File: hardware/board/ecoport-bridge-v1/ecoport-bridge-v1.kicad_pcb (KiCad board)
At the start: 2 copper layers, 51.5 x 92 mm, 68 parts, among them J1 420B2V12FL0, J2 Conn_01x02, J3 SM04B-SRSS-TB, J4 USB4085-GF-A, J5 Conn_01x02, J6 Connector Wire, J7 B3B-PH-K-S, SW1 RESET, SW2 BOOT, U1 IRM-05-5, U2 TLV75733PDBVR, U3 SP3485EET, U4 USBLC6-2SC6, U5 SN74LV1T34DCKR, U6 ESP32-C6-WROOM-1-N8, U7 USBLC6-2SC6

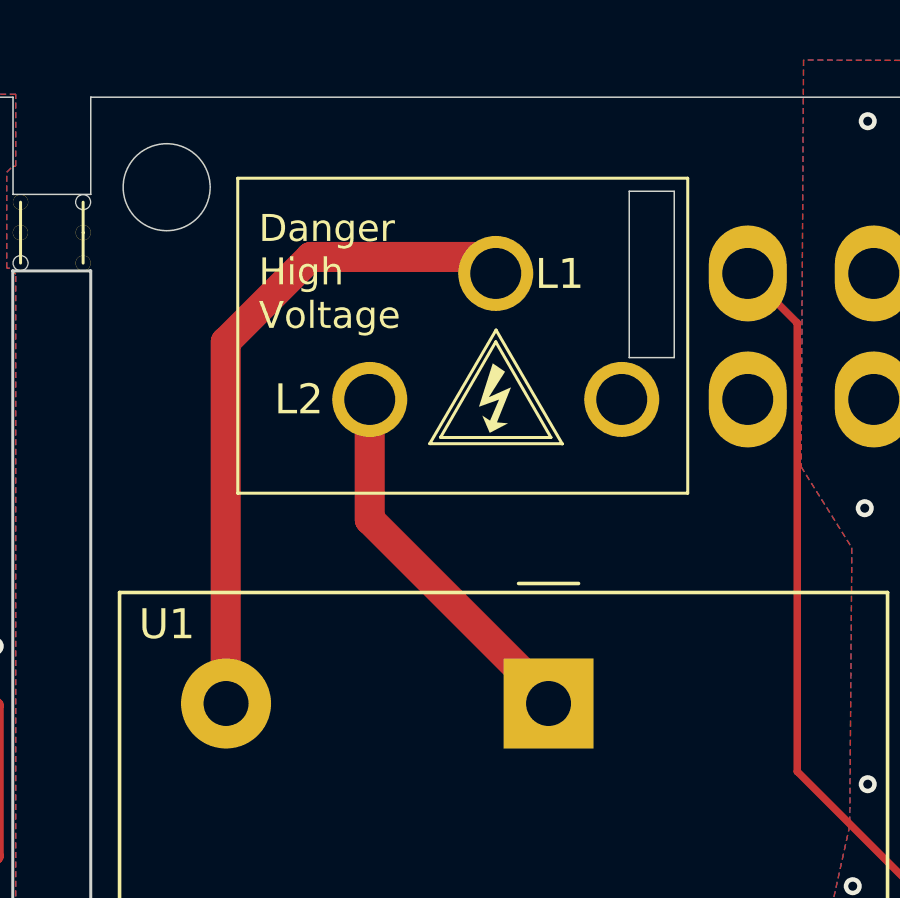
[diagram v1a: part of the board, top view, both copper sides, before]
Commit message: Added fuse
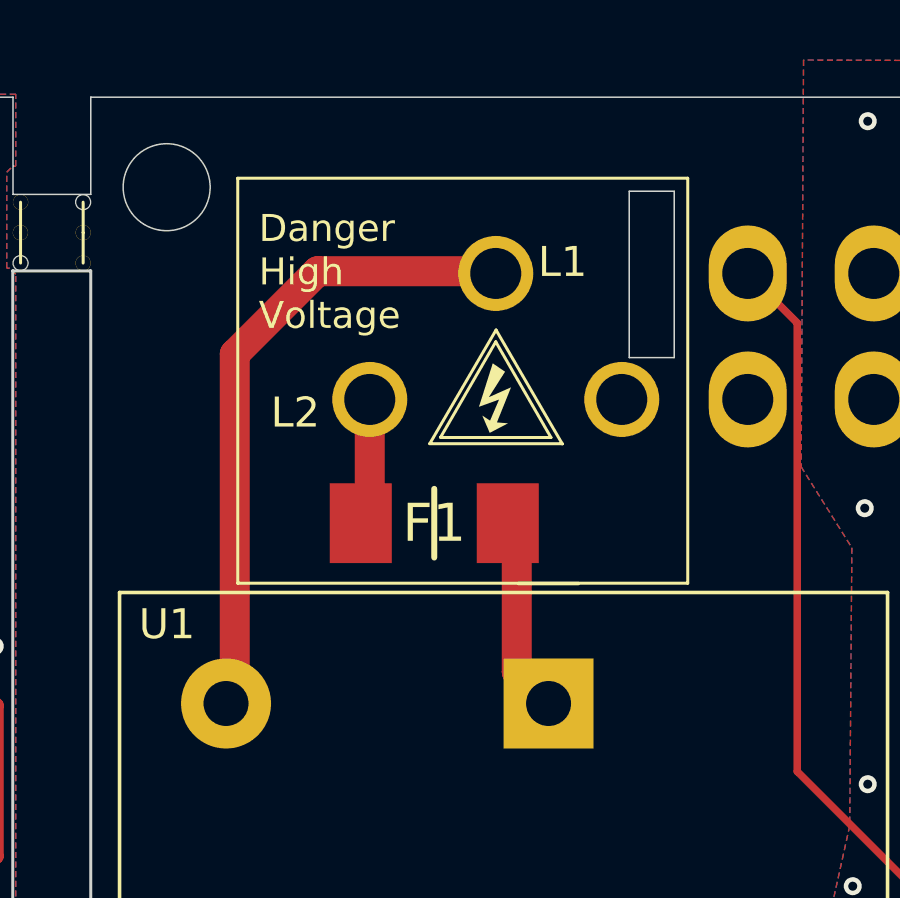
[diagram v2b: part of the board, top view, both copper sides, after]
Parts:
- added F1: SF-2410SP050W-2, Samacsys:FUSC6125X236N, F.Cu at (72.5, 46.4)
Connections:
- U1 pad 1: /AC_L2 -> /AC_L2_F
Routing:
- net /AC_L2: track 12.6 -> 4.31 mm
- net /AC_L2_F: track 0.00 -> 6.34 mm
- net /AC_L1: track 22.5 -> 21.7 mm
